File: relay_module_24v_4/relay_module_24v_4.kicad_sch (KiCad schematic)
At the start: 18 parts, among them J1 Conn_01x12_Pin, J4 Conn_01x05_Pin, K1 Relay_SPDT, K2 Relay_SPDT, K3 Relay_SPDT, K4 Relay_SPDT

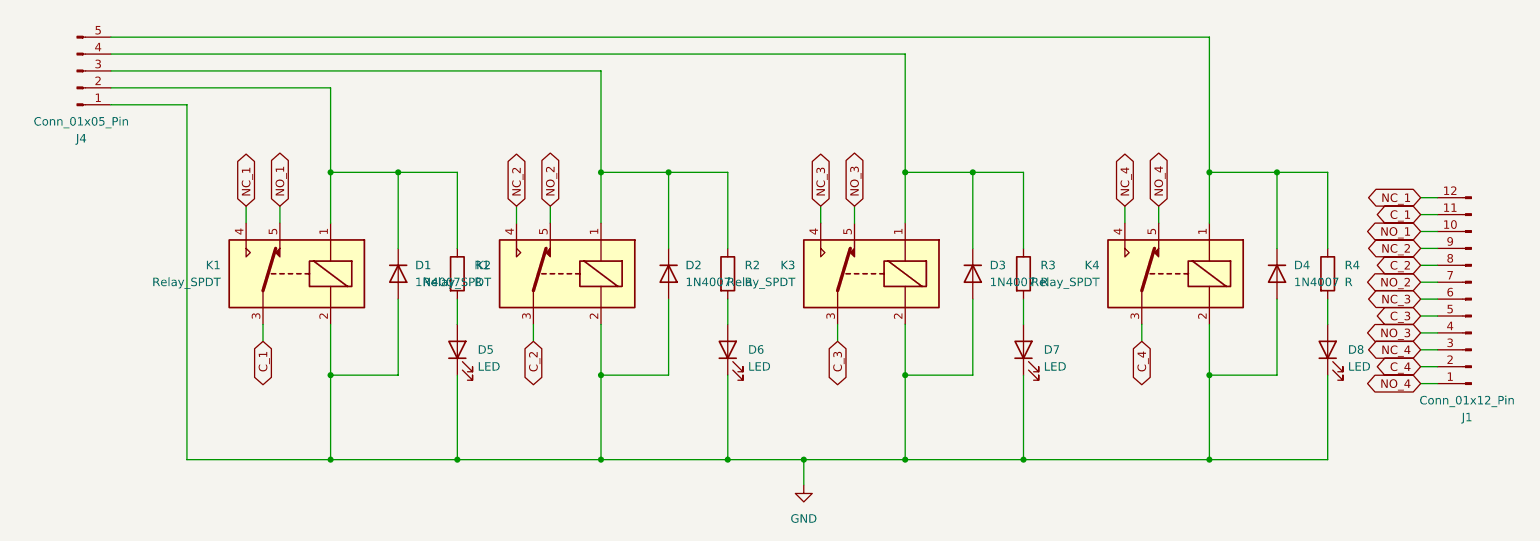
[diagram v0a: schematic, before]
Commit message: v1.0.0
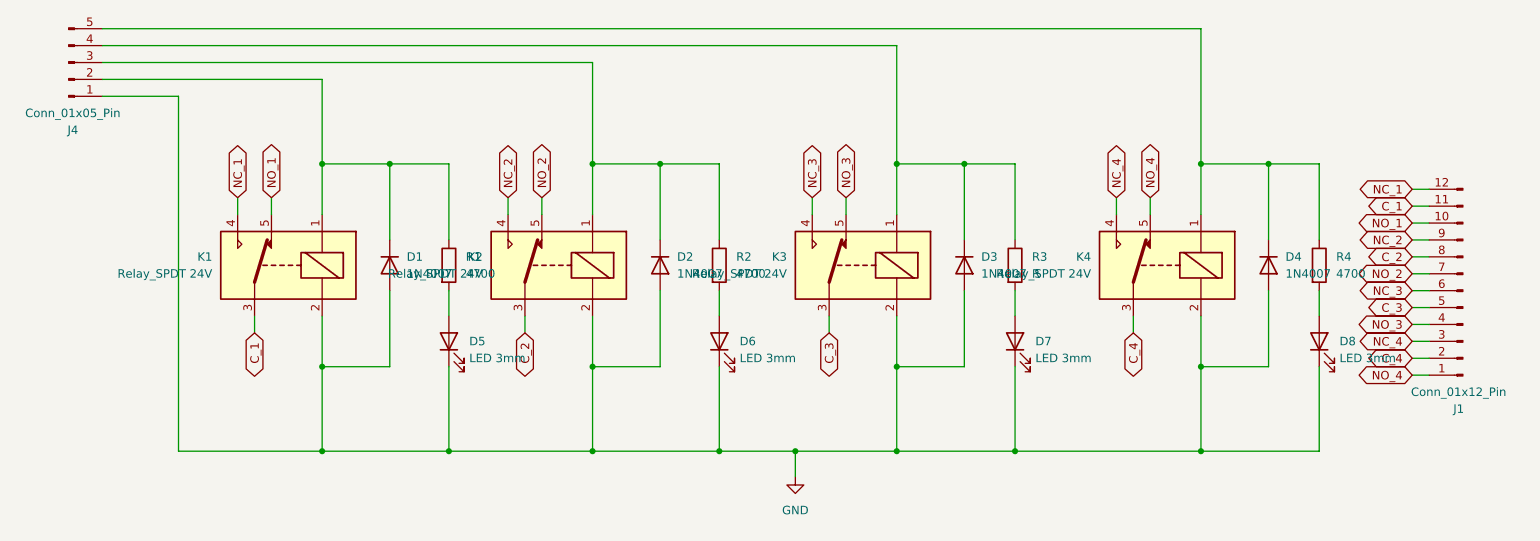
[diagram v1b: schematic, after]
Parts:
- D5, D6, D7, D8: value LED -> LED 3mm
- K1, K2, K3, K4: value Relay_SPDT -> Relay_SPDT 24V
- R1, R2, R4: value R -> 4700
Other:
- moved on the sheet: D1, D2, D3, D4, D5, D6, D7, D8, J1, J4, K1, K2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
